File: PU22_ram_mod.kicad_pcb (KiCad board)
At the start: 2 copper layers, 39.2 x 94.7 mm, 11 parts, among them J1 MOBO, J2 BA8, J3 BA10

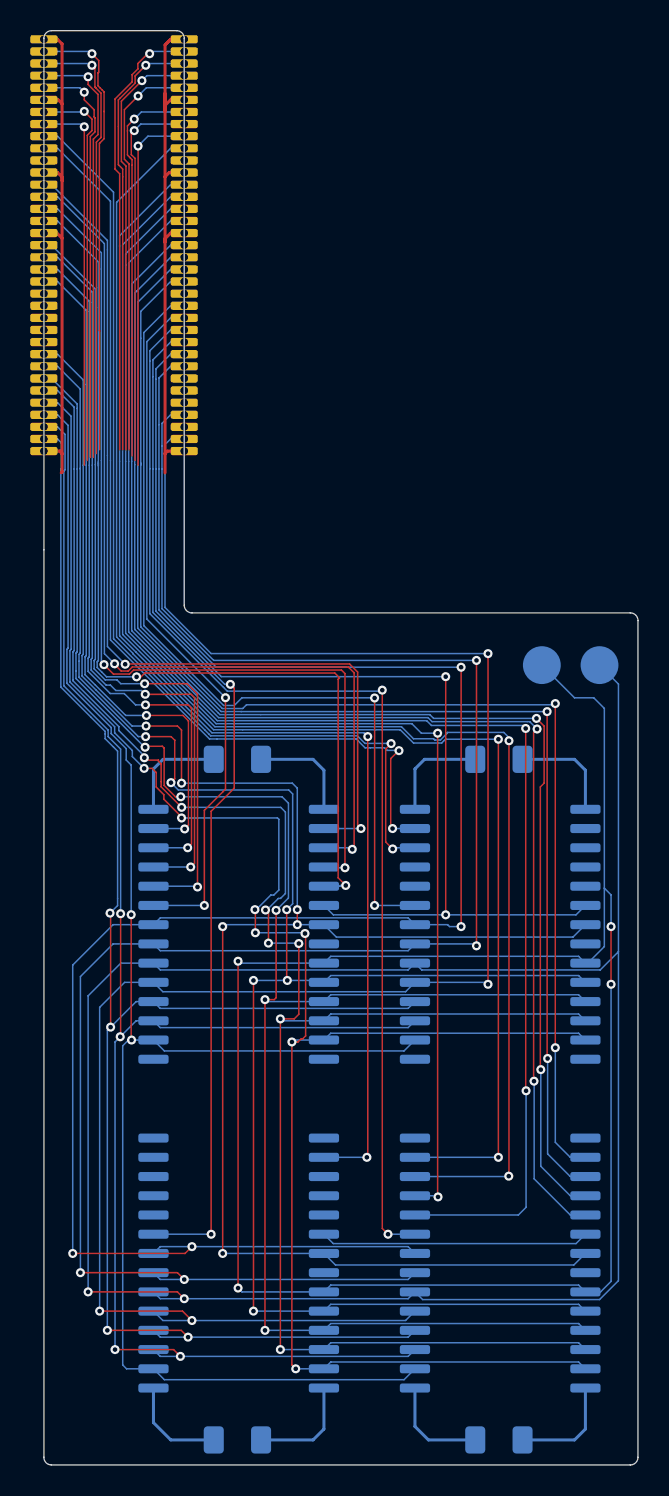
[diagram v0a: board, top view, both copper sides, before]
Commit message: Routing
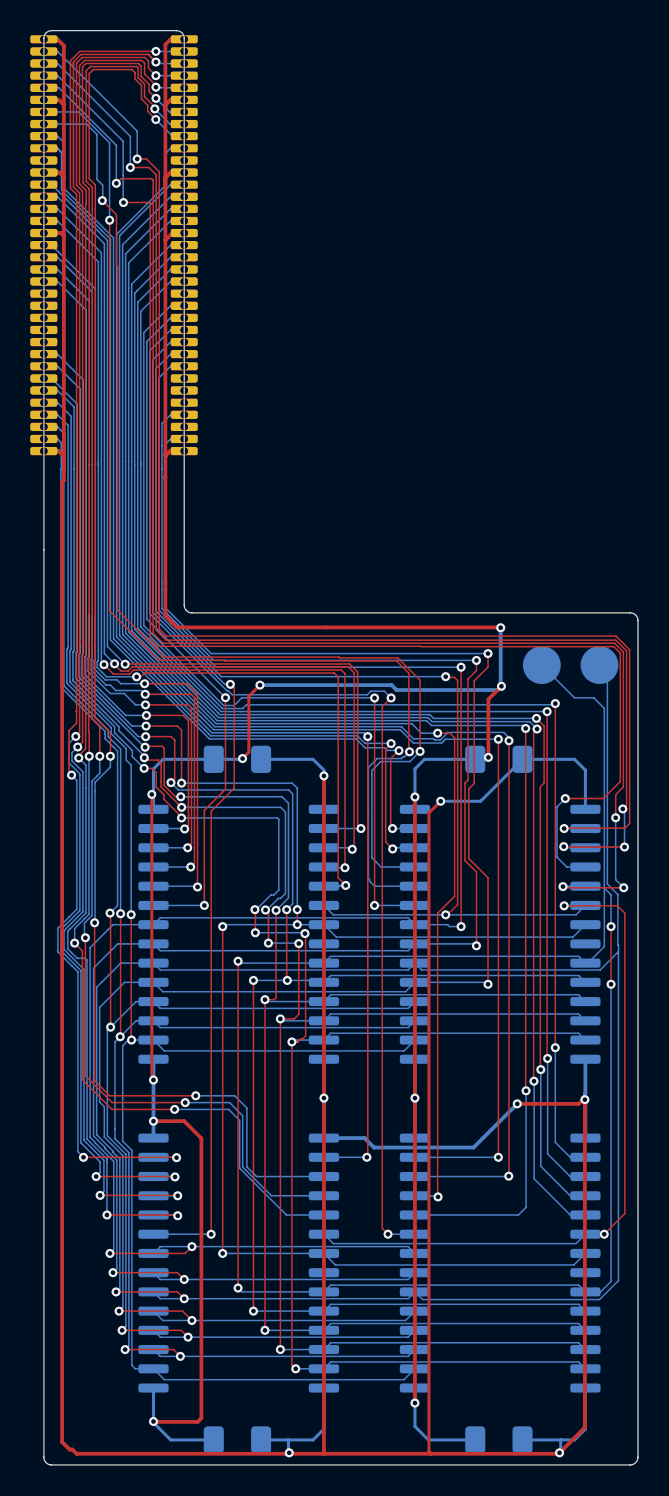
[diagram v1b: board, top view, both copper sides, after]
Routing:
- net VCC: track 63.5 -> 311.1 mm, vias 0 -> 7
- net GND: track 64.6 -> 223.9 mm, vias 0 -> 12
- net /D25: track 24.4 -> 96.8 mm, vias 1 -> 4
- net /D27: track 26.1 -> 98.2 mm, vias 1 -> 4
- net /D26: track 25.5 -> 97.5 mm, vias 1 -> 4
- net /D3: track 27.3 -> 94.5 mm, vias 1 -> 4
- net /D28: track 27.1 -> 93.0 mm, vias 1 -> 4
- net /D29: track 28.0 -> 92.0 mm, vias 1 -> 4
- net /D2: track 28.5 -> 91.9 mm, vias 1 -> 2
- net /D1: track 29.3 -> 92.0 mm, vias 1 -> 4
- net /D30: track 28.9 -> 91.3 mm, vias 1 -> 4
- net /D0: track 29.9 -> 91.2 mm, vias 1 -> 2
- net /D31: track 29.7 -> 90.0 mm, vias 1 -> 4
- net /D4: track 26.1 -> 76.7 mm, vias 1 -> 2
- net /D5: track 25.1 -> 75.0 mm, vias 1 -> 2
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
